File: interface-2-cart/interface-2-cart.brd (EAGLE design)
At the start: 45 x 40.7 mm, 44 parts, among them U3 W25Q128JVSIQ, U4 SN74LVC245ADBR, U5 SN74LVC245ADBR, U6 SN74LVCC4245APWR, X2 TSX-32250, X3 DNP

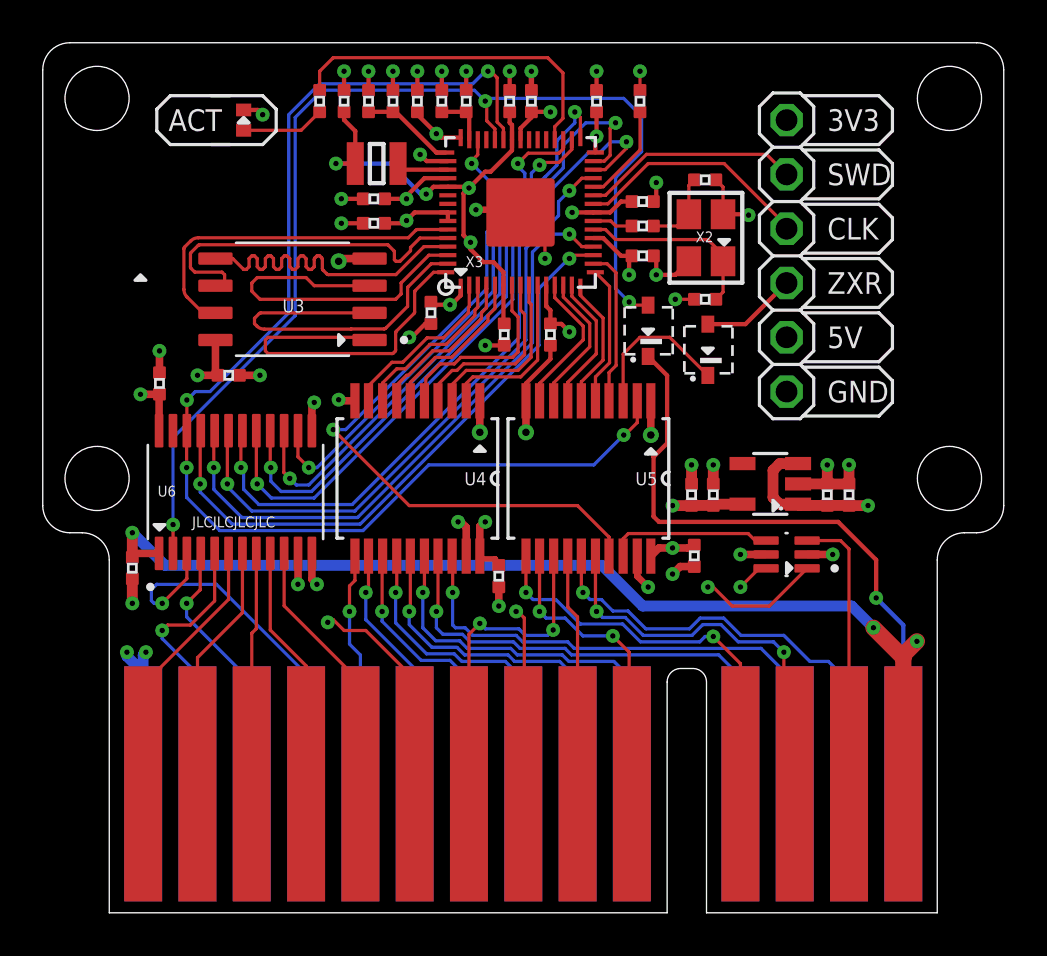
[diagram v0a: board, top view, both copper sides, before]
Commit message: PCB design completed and submitted for production
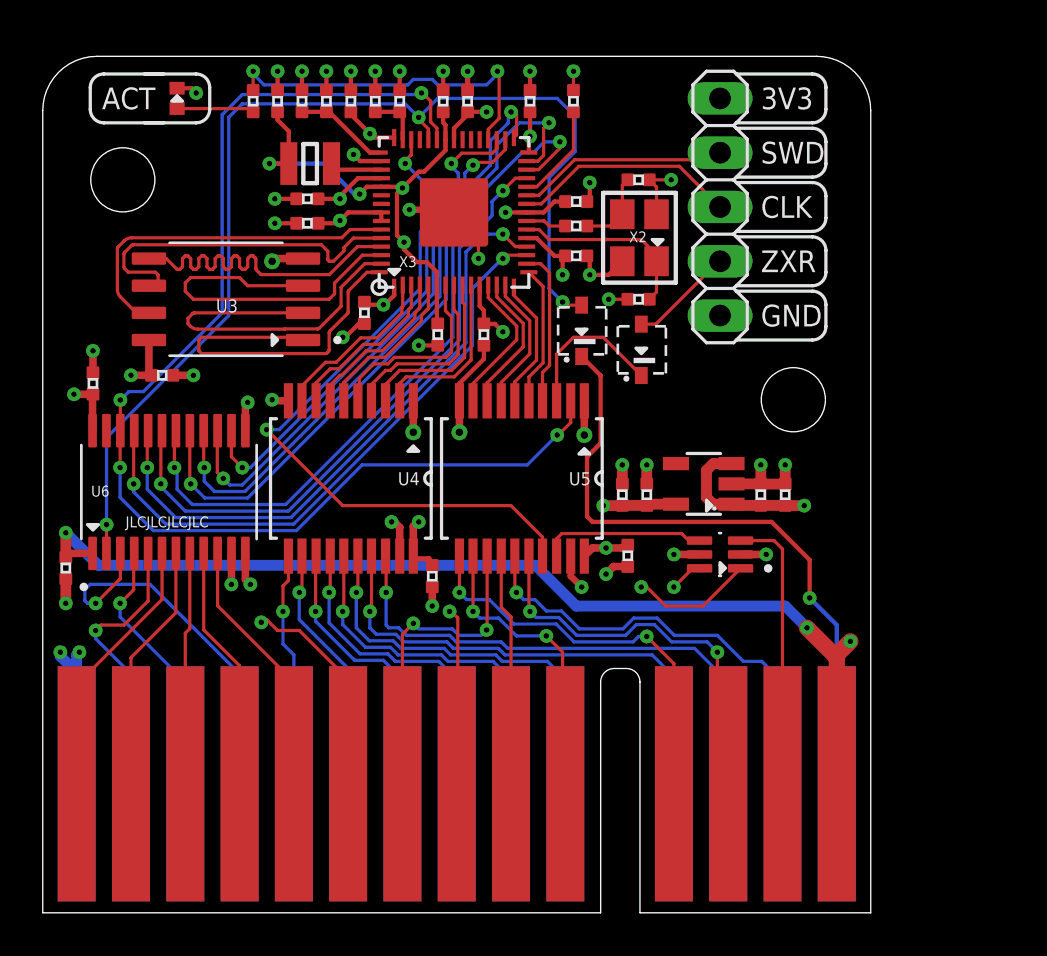
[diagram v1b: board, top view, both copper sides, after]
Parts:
- removed PROG: (no value), adafruit:1X06
- added JP2: (no value), pinhead:1X05
- moved S_LED10 3.27 mm to (6.29, 38.1)
- moved C26 3.24 mm to (27.1, 19.6)
- moved 3V3_REG2 3.11 mm to (30.9, 20.1)
- moved D2 3.11 mm to (25.2, 27.2)
- moved R24 3.11 mm to (24.8, 38.0)
- moved U$2 3.11 mm to (31.7, 16.8)
- moved C19 3.11 mm to (15.0, 28.1)
- moved C24 3.11 mm to (15.6, 38.0)
- moved L1 3.11 mm to (12.5, 35.1)
- moved R20 3.11 mm to (9.84, 38.0)
- moved C12 3.11 mm to (2.35, 24.8)
- moved C18 3.11 mm to (5.59, 25.1)
- moved C2 3.11 mm to (1.08, 16.1)
- moved C1 3.11 mm to (25.0, 33.3)
- moved C10 3.11 mm to (12.4, 33.4)
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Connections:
- net /RESET: now also JP2.4; no longer PROG.4
- net 3V3: now also JP2.1; no longer PROG.1
- net GND: now also JP2.5; no longer PROG.6
- net SWCLK: now also JP2.3; no longer PROG.3
- net SWD: now also JP2.2; no longer PROG.2
- net VCC: no longer PROG.5
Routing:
- net ROMRQ_3V3: track 58.9 -> 57.4 mm
- net /ROMCS_3V3: track 52.5 -> 51.8 mm
- net SWCLK: track 11.2 -> 10.6 mm
- net USER_LED: track 16.1 -> 16.7 mm, vias 0 -> 2
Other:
- board size 45 x 40.7 mm -> 38.7 x 40.1 mm
- board text added: "ZXelerator V1.0 2025 Smashcat"
- board text removed: "5V"
- board text removed: "ZXelerator 2025 Smashcat"
